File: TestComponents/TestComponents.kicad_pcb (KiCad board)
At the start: 2 copper layers, 101.7 x 73.7 mm, 119 parts, among them J2-1 Conn_01x04_Male, J2-2 Conn_01x04_Male, J3V1 Conn_01x01_Male, J5 RFShield_OnePiece, J6 RFShield_OnePiece, SW1 SW_SPDT, SW2 SW_SP3T, SW3 SW_SP3T, U1 AD7991, U13 X, U2 ADS1219, U3 REF200AU, U4 MCP6L01x-xLT, U8 ADR510, U9 LM4040B

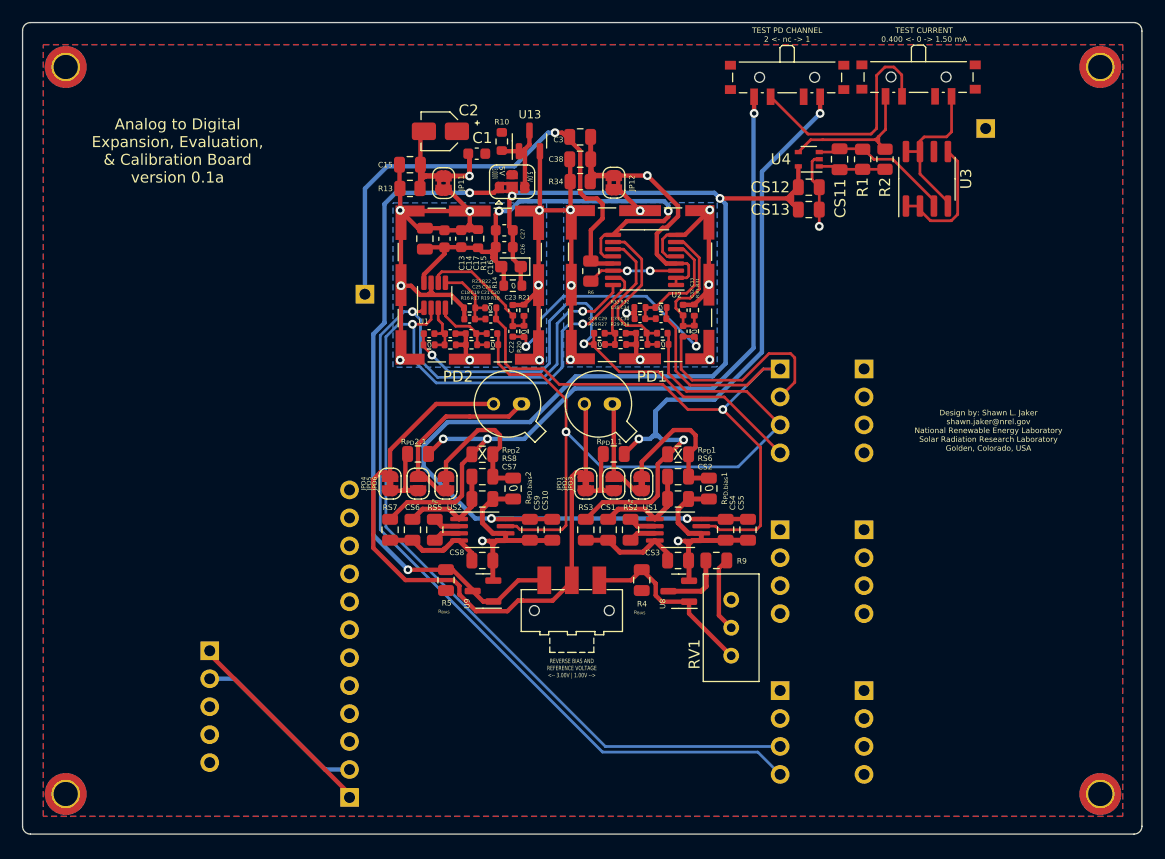
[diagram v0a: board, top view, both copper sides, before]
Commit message: SpectDrone Development
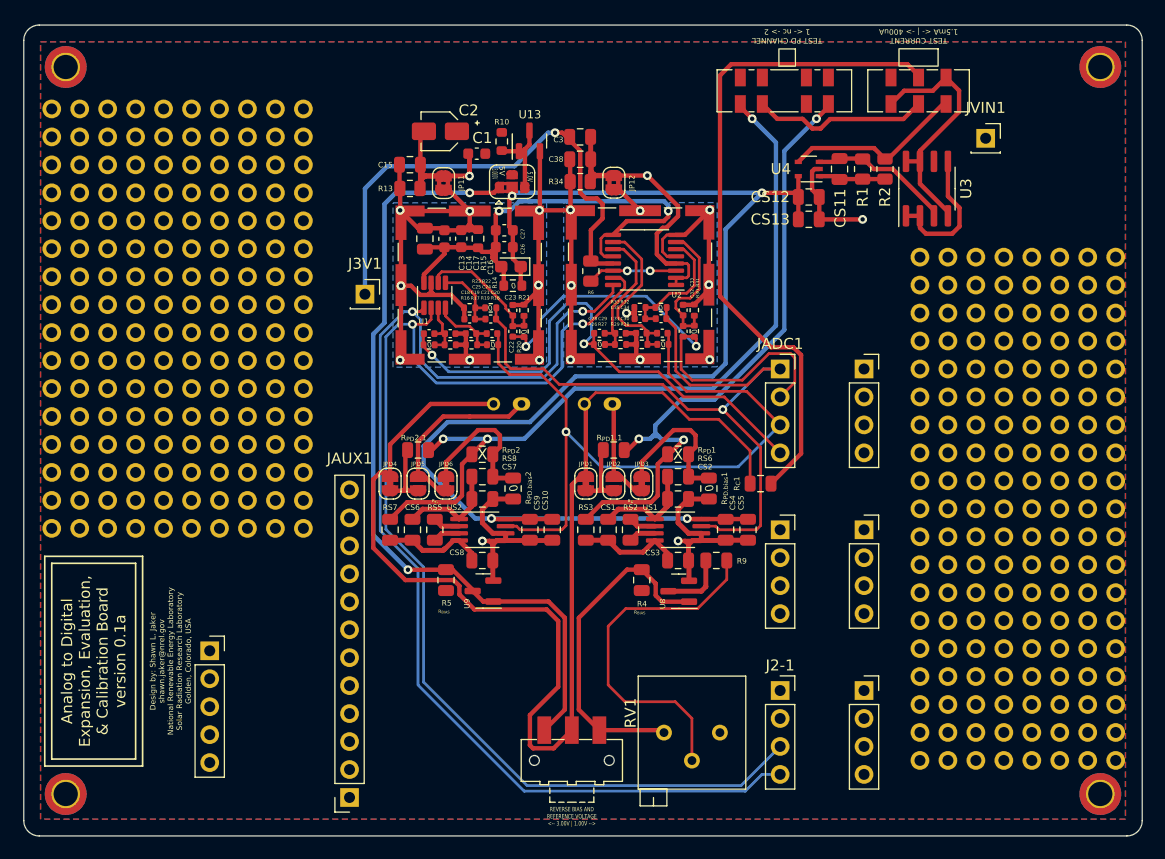
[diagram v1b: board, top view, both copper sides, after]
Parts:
- added REF**: TestPoint_THTPad_D2.0mm_Drill1.0mm, TestPoint:TestPoint_THTPad_D2.0mm_Drill1.0mm, F.Cu at (105.4, 73.7)
- added REF**: TestPoint_THTPad_D2.0mm_Drill1.0mm, TestPoint:TestPoint_THTPad_D2.0mm_Drill1.0mm, F.Cu at (184.3, 87.1)
- added REF**1: TestPoint_THTPad_D2.0mm_Drill1.0mm, TestPoint:TestPoint_THTPad_D2.0mm_Drill1.0mm, F.Cu at (108.0, 73.7)
- added REF**10: TestPoint_THTPad_D2.0mm_Drill1.0mm, TestPoint:TestPoint_THTPad_D2.0mm_Drill1.0mm, F.Cu at (105.4, 76.2)
- added REF**100: TestPoint_THTPad_D2.0mm_Drill1.0mm, TestPoint:TestPoint_THTPad_D2.0mm_Drill1.0mm, F.Cu at (105.4, 99.1)
- added REF**101: TestPoint_THTPad_D2.0mm_Drill1.0mm, TestPoint:TestPoint_THTPad_D2.0mm_Drill1.0mm, F.Cu at (108.0, 99.1)
- added REF**102: TestPoint_THTPad_D2.0mm_Drill1.0mm, TestPoint:TestPoint_THTPad_D2.0mm_Drill1.0mm, F.Cu at (110.5, 99.1)
- added REF**103: TestPoint_THTPad_D2.0mm_Drill1.0mm, TestPoint:TestPoint_THTPad_D2.0mm_Drill1.0mm, F.Cu at (113.0, 99.1)
- added REF**104: TestPoint_THTPad_D2.0mm_Drill1.0mm, TestPoint:TestPoint_THTPad_D2.0mm_Drill1.0mm, F.Cu at (115.6, 99.1)
- added REF**105: TestPoint_THTPad_D2.0mm_Drill1.0mm, TestPoint:TestPoint_THTPad_D2.0mm_Drill1.0mm, F.Cu at (118.1, 99.1)
- added REF**106: TestPoint_THTPad_D2.0mm_Drill1.0mm, TestPoint:TestPoint_THTPad_D2.0mm_Drill1.0mm, F.Cu at (120.7, 99.1)
- added REF**107: TestPoint_THTPad_D2.0mm_Drill1.0mm, TestPoint:TestPoint_THTPad_D2.0mm_Drill1.0mm, F.Cu at (123.2, 99.1)
- added REF**108: TestPoint_THTPad_D2.0mm_Drill1.0mm, TestPoint:TestPoint_THTPad_D2.0mm_Drill1.0mm, F.Cu at (125.7, 99.1)
- added REF**109: TestPoint_THTPad_D2.0mm_Drill1.0mm, TestPoint:TestPoint_THTPad_D2.0mm_Drill1.0mm, F.Cu at (128.3, 99.1)
- added REF**11: TestPoint_THTPad_D2.0mm_Drill1.0mm, TestPoint:TestPoint_THTPad_D2.0mm_Drill1.0mm, F.Cu at (108.0, 76.2)
- added REF**110: TestPoint_THTPad_D2.0mm_Drill1.0mm, TestPoint:TestPoint_THTPad_D2.0mm_Drill1.0mm, F.Cu at (105.4, 101.6)
- added REF**111: TestPoint_THTPad_D2.0mm_Drill1.0mm, TestPoint:TestPoint_THTPad_D2.0mm_Drill1.0mm, F.Cu at (108.0, 101.6)
- added REF**112: TestPoint_THTPad_D2.0mm_Drill1.0mm, TestPoint:TestPoint_THTPad_D2.0mm_Drill1.0mm, F.Cu at (110.5, 101.6)
- added REF**113: TestPoint_THTPad_D2.0mm_Drill1.0mm, TestPoint:TestPoint_THTPad_D2.0mm_Drill1.0mm, F.Cu at (113.0, 101.6)
- added REF**114: TestPoint_THTPad_D2.0mm_Drill1.0mm, TestPoint:TestPoint_THTPad_D2.0mm_Drill1.0mm, F.Cu at (115.6, 101.6)
- added REF**115: TestPoint_THTPad_D2.0mm_Drill1.0mm, TestPoint:TestPoint_THTPad_D2.0mm_Drill1.0mm, F.Cu at (118.1, 101.6)
- added REF**116: TestPoint_THTPad_D2.0mm_Drill1.0mm, TestPoint:TestPoint_THTPad_D2.0mm_Drill1.0mm, F.Cu at (120.7, 101.6)
- added REF**117: TestPoint_THTPad_D2.0mm_Drill1.0mm, TestPoint:TestPoint_THTPad_D2.0mm_Drill1.0mm, F.Cu at (123.2, 101.6)
- added REF**118: TestPoint_THTPad_D2.0mm_Drill1.0mm, TestPoint:TestPoint_THTPad_D2.0mm_Drill1.0mm, F.Cu at (125.7, 101.6)
- added REF**119: TestPoint_THTPad_D2.0mm_Drill1.0mm, TestPoint:TestPoint_THTPad_D2.0mm_Drill1.0mm, F.Cu at (128.3, 101.6)
- added REF**12: TestPoint_THTPad_D2.0mm_Drill1.0mm, TestPoint:TestPoint_THTPad_D2.0mm_Drill1.0mm, F.Cu at (110.5, 76.2)
- added REF**120: TestPoint_THTPad_D2.0mm_Drill1.0mm, TestPoint:TestPoint_THTPad_D2.0mm_Drill1.0mm, F.Cu at (105.4, 104.1)
- added REF**121: TestPoint_THTPad_D2.0mm_Drill1.0mm, TestPoint:TestPoint_THTPad_D2.0mm_Drill1.0mm, F.Cu at (108.0, 104.1)
- added REF**122: TestPoint_THTPad_D2.0mm_Drill1.0mm, TestPoint:TestPoint_THTPad_D2.0mm_Drill1.0mm, F.Cu at (110.5, 104.1)
- added REF**123: TestPoint_THTPad_D2.0mm_Drill1.0mm, TestPoint:TestPoint_THTPad_D2.0mm_Drill1.0mm, F.Cu at (113.0, 104.1)
- added REF**124: TestPoint_THTPad_D2.0mm_Drill1.0mm, TestPoint:TestPoint_THTPad_D2.0mm_Drill1.0mm, F.Cu at (115.6, 104.1)
- added REF**125: TestPoint_THTPad_D2.0mm_Drill1.0mm, TestPoint:TestPoint_THTPad_D2.0mm_Drill1.0mm, F.Cu at (118.1, 104.1)
- added REF**126: TestPoint_THTPad_D2.0mm_Drill1.0mm, TestPoint:TestPoint_THTPad_D2.0mm_Drill1.0mm, F.Cu at (120.7, 104.1)
- added REF**127: TestPoint_THTPad_D2.0mm_Drill1.0mm, TestPoint:TestPoint_THTPad_D2.0mm_Drill1.0mm, F.Cu at (123.2, 104.1)
- added REF**128: TestPoint_THTPad_D2.0mm_Drill1.0mm, TestPoint:TestPoint_THTPad_D2.0mm_Drill1.0mm, F.Cu at (125.7, 104.1)
- added REF**129: TestPoint_THTPad_D2.0mm_Drill1.0mm, TestPoint:TestPoint_THTPad_D2.0mm_Drill1.0mm, F.Cu at (128.3, 104.1)
- added REF**13: TestPoint_THTPad_D2.0mm_Drill1.0mm, TestPoint:TestPoint_THTPad_D2.0mm_Drill1.0mm, F.Cu at (113.0, 76.2)
- added REF**130: TestPoint_THTPad_D2.0mm_Drill1.0mm, TestPoint:TestPoint_THTPad_D2.0mm_Drill1.0mm, F.Cu at (105.4, 106.7)
- added REF**131: TestPoint_THTPad_D2.0mm_Drill1.0mm, TestPoint:TestPoint_THTPad_D2.0mm_Drill1.0mm, F.Cu at (108.0, 106.7)
- added REF**132: TestPoint_THTPad_D2.0mm_Drill1.0mm, TestPoint:TestPoint_THTPad_D2.0mm_Drill1.0mm, F.Cu at (110.5, 106.7)
- added REF**133: TestPoint_THTPad_D2.0mm_Drill1.0mm, TestPoint:TestPoint_THTPad_D2.0mm_Drill1.0mm, F.Cu at (113.0, 106.7)
- added REF**134: TestPoint_THTPad_D2.0mm_Drill1.0mm, TestPoint:TestPoint_THTPad_D2.0mm_Drill1.0mm, F.Cu at (115.6, 106.7)
- added REF**135: TestPoint_THTPad_D2.0mm_Drill1.0mm, TestPoint:TestPoint_THTPad_D2.0mm_Drill1.0mm, F.Cu at (118.1, 106.7)
- added REF**136: TestPoint_THTPad_D2.0mm_Drill1.0mm, TestPoint:TestPoint_THTPad_D2.0mm_Drill1.0mm, F.Cu at (120.7, 106.7)
- added REF**137: TestPoint_THTPad_D2.0mm_Drill1.0mm, TestPoint:TestPoint_THTPad_D2.0mm_Drill1.0mm, F.Cu at (123.2, 106.7)
- added REF**138: TestPoint_THTPad_D2.0mm_Drill1.0mm, TestPoint:TestPoint_THTPad_D2.0mm_Drill1.0mm, F.Cu at (125.7, 106.7)
- added REF**139: TestPoint_THTPad_D2.0mm_Drill1.0mm, TestPoint:TestPoint_THTPad_D2.0mm_Drill1.0mm, F.Cu at (128.3, 106.7)
- added REF**14: TestPoint_THTPad_D2.0mm_Drill1.0mm, TestPoint:TestPoint_THTPad_D2.0mm_Drill1.0mm, F.Cu at (115.6, 76.2)
- added REF**140: TestPoint_THTPad_D2.0mm_Drill1.0mm, TestPoint:TestPoint_THTPad_D2.0mm_Drill1.0mm, F.Cu at (105.4, 109.2)
- added REF**141: TestPoint_THTPad_D2.0mm_Drill1.0mm, TestPoint:TestPoint_THTPad_D2.0mm_Drill1.0mm, F.Cu at (108.0, 109.2)
- added REF**142: TestPoint_THTPad_D2.0mm_Drill1.0mm, TestPoint:TestPoint_THTPad_D2.0mm_Drill1.0mm, F.Cu at (110.5, 109.2)
- added REF**143: TestPoint_THTPad_D2.0mm_Drill1.0mm, TestPoint:TestPoint_THTPad_D2.0mm_Drill1.0mm, F.Cu at (113.0, 109.2)
- added REF**144: TestPoint_THTPad_D2.0mm_Drill1.0mm, TestPoint:TestPoint_THTPad_D2.0mm_Drill1.0mm, F.Cu at (115.6, 109.2)
- added REF**145: TestPoint_THTPad_D2.0mm_Drill1.0mm, TestPoint:TestPoint_THTPad_D2.0mm_Drill1.0mm, F.Cu at (118.1, 109.2)
- added REF**146: TestPoint_THTPad_D2.0mm_Drill1.0mm, TestPoint:TestPoint_THTPad_D2.0mm_Drill1.0mm, F.Cu at (120.7, 109.2)
- added REF**147: TestPoint_THTPad_D2.0mm_Drill1.0mm, TestPoint:TestPoint_THTPad_D2.0mm_Drill1.0mm, F.Cu at (123.2, 109.2)
- added REF**148: TestPoint_THTPad_D2.0mm_Drill1.0mm, TestPoint:TestPoint_THTPad_D2.0mm_Drill1.0mm, F.Cu at (125.7, 109.2)
- added REF**149: TestPoint_THTPad_D2.0mm_Drill1.0mm, TestPoint:TestPoint_THTPad_D2.0mm_Drill1.0mm, F.Cu at (128.3, 109.2)
- added REF**15: TestPoint_THTPad_D2.0mm_Drill1.0mm, TestPoint:TestPoint_THTPad_D2.0mm_Drill1.0mm, F.Cu at (118.1, 76.2)
- added REF**150: TestPoint_THTPad_D2.0mm_Drill1.0mm, TestPoint:TestPoint_THTPad_D2.0mm_Drill1.0mm, F.Cu at (105.4, 111.8)
- added REF**151: TestPoint_THTPad_D2.0mm_Drill1.0mm, TestPoint:TestPoint_THTPad_D2.0mm_Drill1.0mm, F.Cu at (108.0, 111.8)
- added REF**152: TestPoint_THTPad_D2.0mm_Drill1.0mm, TestPoint:TestPoint_THTPad_D2.0mm_Drill1.0mm, F.Cu at (110.5, 111.8)
- added REF**153: TestPoint_THTPad_D2.0mm_Drill1.0mm, TestPoint:TestPoint_THTPad_D2.0mm_Drill1.0mm, F.Cu at (113.0, 111.8)
- added REF**154: TestPoint_THTPad_D2.0mm_Drill1.0mm, TestPoint:TestPoint_THTPad_D2.0mm_Drill1.0mm, F.Cu at (115.6, 111.8)
- added REF**155: TestPoint_THTPad_D2.0mm_Drill1.0mm, TestPoint:TestPoint_THTPad_D2.0mm_Drill1.0mm, F.Cu at (118.1, 111.8)
- added REF**156: TestPoint_THTPad_D2.0mm_Drill1.0mm, TestPoint:TestPoint_THTPad_D2.0mm_Drill1.0mm, F.Cu at (120.7, 111.8)
- added REF**157: TestPoint_THTPad_D2.0mm_Drill1.0mm, TestPoint:TestPoint_THTPad_D2.0mm_Drill1.0mm, F.Cu at (123.2, 111.8)
- added REF**158: TestPoint_THTPad_D2.0mm_Drill1.0mm, TestPoint:TestPoint_THTPad_D2.0mm_Drill1.0mm, F.Cu at (125.7, 111.8)
- added REF**159: TestPoint_THTPad_D2.0mm_Drill1.0mm, TestPoint:TestPoint_THTPad_D2.0mm_Drill1.0mm, F.Cu at (128.3, 111.8)
- added REF**16: TestPoint_THTPad_D2.0mm_Drill1.0mm, TestPoint:TestPoint_THTPad_D2.0mm_Drill1.0mm, F.Cu at (120.7, 76.2)
- added REF**160: TestPoint_THTPad_D2.0mm_Drill1.0mm, TestPoint:TestPoint_THTPad_D2.0mm_Drill1.0mm, F.Cu at (186.8, 87.1)
- added REF**161: TestPoint_THTPad_D2.0mm_Drill1.0mm, TestPoint:TestPoint_THTPad_D2.0mm_Drill1.0mm, F.Cu at (189.4, 87.1)
- added REF**162: TestPoint_THTPad_D2.0mm_Drill1.0mm, TestPoint:TestPoint_THTPad_D2.0mm_Drill1.0mm, F.Cu at (191.9, 87.1)
- added REF**163: TestPoint_THTPad_D2.0mm_Drill1.0mm, TestPoint:TestPoint_THTPad_D2.0mm_Drill1.0mm, F.Cu at (194.4, 87.1)
- added REF**164: TestPoint_THTPad_D2.0mm_Drill1.0mm, TestPoint:TestPoint_THTPad_D2.0mm_Drill1.0mm, F.Cu at (197.0, 87.1)
- added REF**165: TestPoint_THTPad_D2.0mm_Drill1.0mm, TestPoint:TestPoint_THTPad_D2.0mm_Drill1.0mm, F.Cu at (199.5, 87.1)
- added REF**166: TestPoint_THTPad_D2.0mm_Drill1.0mm, TestPoint:TestPoint_THTPad_D2.0mm_Drill1.0mm, F.Cu at (202.1, 87.1)
- added REF**167: TestPoint_THTPad_D2.0mm_Drill1.0mm, TestPoint:TestPoint_THTPad_D2.0mm_Drill1.0mm, F.Cu at (184.3, 89.7)
- added REF**168: TestPoint_THTPad_D2.0mm_Drill1.0mm, TestPoint:TestPoint_THTPad_D2.0mm_Drill1.0mm, F.Cu at (186.8, 89.7)
- added REF**169: TestPoint_THTPad_D2.0mm_Drill1.0mm, TestPoint:TestPoint_THTPad_D2.0mm_Drill1.0mm, F.Cu at (189.4, 89.7)
- added REF**17: TestPoint_THTPad_D2.0mm_Drill1.0mm, TestPoint:TestPoint_THTPad_D2.0mm_Drill1.0mm, F.Cu at (123.2, 76.2)
- added REF**170: TestPoint_THTPad_D2.0mm_Drill1.0mm, TestPoint:TestPoint_THTPad_D2.0mm_Drill1.0mm, F.Cu at (191.9, 89.7)
- added REF**171: TestPoint_THTPad_D2.0mm_Drill1.0mm, TestPoint:TestPoint_THTPad_D2.0mm_Drill1.0mm, F.Cu at (194.4, 89.7)
- added REF**172: TestPoint_THTPad_D2.0mm_Drill1.0mm, TestPoint:TestPoint_THTPad_D2.0mm_Drill1.0mm, F.Cu at (197.0, 89.7)
- added REF**173: TestPoint_THTPad_D2.0mm_Drill1.0mm, TestPoint:TestPoint_THTPad_D2.0mm_Drill1.0mm, F.Cu at (199.5, 89.7)
- added REF**174: TestPoint_THTPad_D2.0mm_Drill1.0mm, TestPoint:TestPoint_THTPad_D2.0mm_Drill1.0mm, F.Cu at (202.1, 89.7)
- added REF**175: TestPoint_THTPad_D2.0mm_Drill1.0mm, TestPoint:TestPoint_THTPad_D2.0mm_Drill1.0mm, F.Cu at (184.3, 92.2)
- added REF**176: TestPoint_THTPad_D2.0mm_Drill1.0mm, TestPoint:TestPoint_THTPad_D2.0mm_Drill1.0mm, F.Cu at (186.8, 92.2)
- added REF**177: TestPoint_THTPad_D2.0mm_Drill1.0mm, TestPoint:TestPoint_THTPad_D2.0mm_Drill1.0mm, F.Cu at (189.4, 92.2)
- added REF**178: TestPoint_THTPad_D2.0mm_Drill1.0mm, TestPoint:TestPoint_THTPad_D2.0mm_Drill1.0mm, F.Cu at (191.9, 92.2)
- added REF**179: TestPoint_THTPad_D2.0mm_Drill1.0mm, TestPoint:TestPoint_THTPad_D2.0mm_Drill1.0mm, F.Cu at (194.4, 92.2)
- added REF**18: TestPoint_THTPad_D2.0mm_Drill1.0mm, TestPoint:TestPoint_THTPad_D2.0mm_Drill1.0mm, F.Cu at (125.7, 76.2)
- added REF**180: TestPoint_THTPad_D2.0mm_Drill1.0mm, TestPoint:TestPoint_THTPad_D2.0mm_Drill1.0mm, F.Cu at (197.0, 92.2)
- added REF**181: TestPoint_THTPad_D2.0mm_Drill1.0mm, TestPoint:TestPoint_THTPad_D2.0mm_Drill1.0mm, F.Cu at (199.5, 92.2)
- added REF**182: TestPoint_THTPad_D2.0mm_Drill1.0mm, TestPoint:TestPoint_THTPad_D2.0mm_Drill1.0mm, F.Cu at (202.1, 92.2)
- added REF**183: TestPoint_THTPad_D2.0mm_Drill1.0mm, TestPoint:TestPoint_THTPad_D2.0mm_Drill1.0mm, F.Cu at (184.3, 94.7)
- added REF**184: TestPoint_THTPad_D2.0mm_Drill1.0mm, TestPoint:TestPoint_THTPad_D2.0mm_Drill1.0mm, F.Cu at (186.8, 94.7)
- added REF**185: TestPoint_THTPad_D2.0mm_Drill1.0mm, TestPoint:TestPoint_THTPad_D2.0mm_Drill1.0mm, F.Cu at (189.4, 94.7)
- added REF**186: TestPoint_THTPad_D2.0mm_Drill1.0mm, TestPoint:TestPoint_THTPad_D2.0mm_Drill1.0mm, F.Cu at (191.9, 94.7)
- added REF**187: TestPoint_THTPad_D2.0mm_Drill1.0mm, TestPoint:TestPoint_THTPad_D2.0mm_Drill1.0mm, F.Cu at (194.4, 94.7)
- added REF**188: TestPoint_THTPad_D2.0mm_Drill1.0mm, TestPoint:TestPoint_THTPad_D2.0mm_Drill1.0mm, F.Cu at (197.0, 94.7)
- added REF**189: TestPoint_THTPad_D2.0mm_Drill1.0mm, TestPoint:TestPoint_THTPad_D2.0mm_Drill1.0mm, F.Cu at (199.5, 94.7)
- added REF**19: TestPoint_THTPad_D2.0mm_Drill1.0mm, TestPoint:TestPoint_THTPad_D2.0mm_Drill1.0mm, F.Cu at (128.3, 76.2)
- added REF**190: TestPoint_THTPad_D2.0mm_Drill1.0mm, TestPoint:TestPoint_THTPad_D2.0mm_Drill1.0mm, F.Cu at (202.1, 94.7)
- added REF**191: TestPoint_THTPad_D2.0mm_Drill1.0mm, TestPoint:TestPoint_THTPad_D2.0mm_Drill1.0mm, F.Cu at (184.3, 97.3)
- added REF**192: TestPoint_THTPad_D2.0mm_Drill1.0mm, TestPoint:TestPoint_THTPad_D2.0mm_Drill1.0mm, F.Cu at (186.8, 97.3)
- added REF**193: TestPoint_THTPad_D2.0mm_Drill1.0mm, TestPoint:TestPoint_THTPad_D2.0mm_Drill1.0mm, F.Cu at (189.4, 97.3)
- added REF**194: TestPoint_THTPad_D2.0mm_Drill1.0mm, TestPoint:TestPoint_THTPad_D2.0mm_Drill1.0mm, F.Cu at (191.9, 97.3)
- added REF**195: TestPoint_THTPad_D2.0mm_Drill1.0mm, TestPoint:TestPoint_THTPad_D2.0mm_Drill1.0mm, F.Cu at (194.4, 97.3)
- added REF**196: TestPoint_THTPad_D2.0mm_Drill1.0mm, TestPoint:TestPoint_THTPad_D2.0mm_Drill1.0mm, F.Cu at (197.0, 97.3)
- added REF**197: TestPoint_THTPad_D2.0mm_Drill1.0mm, TestPoint:TestPoint_THTPad_D2.0mm_Drill1.0mm, F.Cu at (199.5, 97.3)
- added REF**198: TestPoint_THTPad_D2.0mm_Drill1.0mm, TestPoint:TestPoint_THTPad_D2.0mm_Drill1.0mm, F.Cu at (202.1, 97.3)
- added REF**199: TestPoint_THTPad_D2.0mm_Drill1.0mm, TestPoint:TestPoint_THTPad_D2.0mm_Drill1.0mm, F.Cu at (184.3, 99.8)
- added REF**2: TestPoint_THTPad_D2.0mm_Drill1.0mm, TestPoint:TestPoint_THTPad_D2.0mm_Drill1.0mm, F.Cu at (110.5, 73.7)
- added REF**20: TestPoint_THTPad_D2.0mm_Drill1.0mm, TestPoint:TestPoint_THTPad_D2.0mm_Drill1.0mm, F.Cu at (105.4, 78.7)
- added REF**200: TestPoint_THTPad_D2.0mm_Drill1.0mm, TestPoint:TestPoint_THTPad_D2.0mm_Drill1.0mm, F.Cu at (186.8, 99.8)
- added REF**201: TestPoint_THTPad_D2.0mm_Drill1.0mm, TestPoint:TestPoint_THTPad_D2.0mm_Drill1.0mm, F.Cu at (189.4, 99.8)
- added REF**202: TestPoint_THTPad_D2.0mm_Drill1.0mm, TestPoint:TestPoint_THTPad_D2.0mm_Drill1.0mm, F.Cu at (191.9, 99.8)
- added REF**203: TestPoint_THTPad_D2.0mm_Drill1.0mm, TestPoint:TestPoint_THTPad_D2.0mm_Drill1.0mm, F.Cu at (194.4, 99.8)
- added REF**204: TestPoint_THTPad_D2.0mm_Drill1.0mm, TestPoint:TestPoint_THTPad_D2.0mm_Drill1.0mm, F.Cu at (197.0, 99.8)
- added REF**205: TestPoint_THTPad_D2.0mm_Drill1.0mm, TestPoint:TestPoint_THTPad_D2.0mm_Drill1.0mm, F.Cu at (199.5, 99.8)
- added REF**206: TestPoint_THTPad_D2.0mm_Drill1.0mm, TestPoint:TestPoint_THTPad_D2.0mm_Drill1.0mm, F.Cu at (202.1, 99.8)
- added REF**207: TestPoint_THTPad_D2.0mm_Drill1.0mm, TestPoint:TestPoint_THTPad_D2.0mm_Drill1.0mm, F.Cu at (184.3, 102.4)
- added REF**208: TestPoint_THTPad_D2.0mm_Drill1.0mm, TestPoint:TestPoint_THTPad_D2.0mm_Drill1.0mm, F.Cu at (186.8, 102.4)
- added REF**209: TestPoint_THTPad_D2.0mm_Drill1.0mm, TestPoint:TestPoint_THTPad_D2.0mm_Drill1.0mm, F.Cu at (189.4, 102.4)
- added REF**21: TestPoint_THTPad_D2.0mm_Drill1.0mm, TestPoint:TestPoint_THTPad_D2.0mm_Drill1.0mm, F.Cu at (108.0, 78.7)
- added REF**210: TestPoint_THTPad_D2.0mm_Drill1.0mm, TestPoint:TestPoint_THTPad_D2.0mm_Drill1.0mm, F.Cu at (191.9, 102.4)
- added REF**211: TestPoint_THTPad_D2.0mm_Drill1.0mm, TestPoint:TestPoint_THTPad_D2.0mm_Drill1.0mm, F.Cu at (194.4, 102.4)
- added REF**212: TestPoint_THTPad_D2.0mm_Drill1.0mm, TestPoint:TestPoint_THTPad_D2.0mm_Drill1.0mm, F.Cu at (197.0, 102.4)
- added REF**213: TestPoint_THTPad_D2.0mm_Drill1.0mm, TestPoint:TestPoint_THTPad_D2.0mm_Drill1.0mm, F.Cu at (199.5, 102.4)
- added REF**214: TestPoint_THTPad_D2.0mm_Drill1.0mm, TestPoint:TestPoint_THTPad_D2.0mm_Drill1.0mm, F.Cu at (202.1, 102.4)
- added REF**215: TestPoint_THTPad_D2.0mm_Drill1.0mm, TestPoint:TestPoint_THTPad_D2.0mm_Drill1.0mm, F.Cu at (184.3, 104.9)
- added REF**216: TestPoint_THTPad_D2.0mm_Drill1.0mm, TestPoint:TestPoint_THTPad_D2.0mm_Drill1.0mm, F.Cu at (186.8, 104.9)
- added REF**217: TestPoint_THTPad_D2.0mm_Drill1.0mm, TestPoint:TestPoint_THTPad_D2.0mm_Drill1.0mm, F.Cu at (189.4, 104.9)
- added REF**218: TestPoint_THTPad_D2.0mm_Drill1.0mm, TestPoint:TestPoint_THTPad_D2.0mm_Drill1.0mm, F.Cu at (191.9, 104.9)
- added REF**219: TestPoint_THTPad_D2.0mm_Drill1.0mm, TestPoint:TestPoint_THTPad_D2.0mm_Drill1.0mm, F.Cu at (194.4, 104.9)
- added REF**22: TestPoint_THTPad_D2.0mm_Drill1.0mm, TestPoint:TestPoint_THTPad_D2.0mm_Drill1.0mm, F.Cu at (110.5, 78.7)
- added REF**220: TestPoint_THTPad_D2.0mm_Drill1.0mm, TestPoint:TestPoint_THTPad_D2.0mm_Drill1.0mm, F.Cu at (197.0, 104.9)
- added REF**221: TestPoint_THTPad_D2.0mm_Drill1.0mm, TestPoint:TestPoint_THTPad_D2.0mm_Drill1.0mm, F.Cu at (199.5, 104.9)
- added REF**222: TestPoint_THTPad_D2.0mm_Drill1.0mm, TestPoint:TestPoint_THTPad_D2.0mm_Drill1.0mm, F.Cu at (202.1, 104.9)
- added REF**223: TestPoint_THTPad_D2.0mm_Drill1.0mm, TestPoint:TestPoint_THTPad_D2.0mm_Drill1.0mm, F.Cu at (184.3, 107.4)
- added REF**224: TestPoint_THTPad_D2.0mm_Drill1.0mm, TestPoint:TestPoint_THTPad_D2.0mm_Drill1.0mm, F.Cu at (186.8, 107.4)
- added REF**225: TestPoint_THTPad_D2.0mm_Drill1.0mm, TestPoint:TestPoint_THTPad_D2.0mm_Drill1.0mm, F.Cu at (189.4, 107.4)
- added REF**226: TestPoint_THTPad_D2.0mm_Drill1.0mm, TestPoint:TestPoint_THTPad_D2.0mm_Drill1.0mm, F.Cu at (191.9, 107.4)
- added REF**227: TestPoint_THTPad_D2.0mm_Drill1.0mm, TestPoint:TestPoint_THTPad_D2.0mm_Drill1.0mm, F.Cu at (194.4, 107.4)
- added REF**228: TestPoint_THTPad_D2.0mm_Drill1.0mm, TestPoint:TestPoint_THTPad_D2.0mm_Drill1.0mm, F.Cu at (197.0, 107.4)
- added REF**229: TestPoint_THTPad_D2.0mm_Drill1.0mm, TestPoint:TestPoint_THTPad_D2.0mm_Drill1.0mm, F.Cu at (199.5, 107.4)
- added REF**23: TestPoint_THTPad_D2.0mm_Drill1.0mm, TestPoint:TestPoint_THTPad_D2.0mm_Drill1.0mm, F.Cu at (113.0, 78.7)
- added REF**230: TestPoint_THTPad_D2.0mm_Drill1.0mm, TestPoint:TestPoint_THTPad_D2.0mm_Drill1.0mm, F.Cu at (202.1, 107.4)
- added REF**231: TestPoint_THTPad_D2.0mm_Drill1.0mm, TestPoint:TestPoint_THTPad_D2.0mm_Drill1.0mm, F.Cu at (184.3, 110.0)
- added REF**232: TestPoint_THTPad_D2.0mm_Drill1.0mm, TestPoint:TestPoint_THTPad_D2.0mm_Drill1.0mm, F.Cu at (186.8, 110.0)
- added REF**233: TestPoint_THTPad_D2.0mm_Drill1.0mm, TestPoint:TestPoint_THTPad_D2.0mm_Drill1.0mm, F.Cu at (189.4, 110.0)
- added REF**234: TestPoint_THTPad_D2.0mm_Drill1.0mm, TestPoint:TestPoint_THTPad_D2.0mm_Drill1.0mm, F.Cu at (191.9, 110.0)
- added REF**235: TestPoint_THTPad_D2.0mm_Drill1.0mm, TestPoint:TestPoint_THTPad_D2.0mm_Drill1.0mm, F.Cu at (194.4, 110.0)
- added REF**236: TestPoint_THTPad_D2.0mm_Drill1.0mm, TestPoint:TestPoint_THTPad_D2.0mm_Drill1.0mm, F.Cu at (197.0, 110.0)
- added REF**237: TestPoint_THTPad_D2.0mm_Drill1.0mm, TestPoint:TestPoint_THTPad_D2.0mm_Drill1.0mm, F.Cu at (199.5, 110.0)
- added REF**238: TestPoint_THTPad_D2.0mm_Drill1.0mm, TestPoint:TestPoint_THTPad_D2.0mm_Drill1.0mm, F.Cu at (202.1, 110.0)
- added REF**239: TestPoint_THTPad_D2.0mm_Drill1.0mm, TestPoint:TestPoint_THTPad_D2.0mm_Drill1.0mm, F.Cu at (184.3, 112.5)
- added REF**24: TestPoint_THTPad_D2.0mm_Drill1.0mm, TestPoint:TestPoint_THTPad_D2.0mm_Drill1.0mm, F.Cu at (115.6, 78.7)
- added REF**240: TestPoint_THTPad_D2.0mm_Drill1.0mm, TestPoint:TestPoint_THTPad_D2.0mm_Drill1.0mm, F.Cu at (186.8, 112.5)
- added REF**241: TestPoint_THTPad_D2.0mm_Drill1.0mm, TestPoint:TestPoint_THTPad_D2.0mm_Drill1.0mm, F.Cu at (189.4, 112.5)
- added REF**242: TestPoint_THTPad_D2.0mm_Drill1.0mm, TestPoint:TestPoint_THTPad_D2.0mm_Drill1.0mm, F.Cu at (191.9, 112.5)
- added REF**243: TestPoint_THTPad_D2.0mm_Drill1.0mm, TestPoint:TestPoint_THTPad_D2.0mm_Drill1.0mm, F.Cu at (194.4, 112.5)
- added REF**244: TestPoint_THTPad_D2.0mm_Drill1.0mm, TestPoint:TestPoint_THTPad_D2.0mm_Drill1.0mm, F.Cu at (197.0, 112.5)
- added REF**245: TestPoint_THTPad_D2.0mm_Drill1.0mm, TestPoint:TestPoint_THTPad_D2.0mm_Drill1.0mm, F.Cu at (199.5, 112.5)
- added REF**246: TestPoint_THTPad_D2.0mm_Drill1.0mm, TestPoint:TestPoint_THTPad_D2.0mm_Drill1.0mm, F.Cu at (202.1, 112.5)
- added REF**247: TestPoint_THTPad_D2.0mm_Drill1.0mm, TestPoint:TestPoint_THTPad_D2.0mm_Drill1.0mm, F.Cu at (184.3, 115.1)
- added REF**248: TestPoint_THTPad_D2.0mm_Drill1.0mm, TestPoint:TestPoint_THTPad_D2.0mm_Drill1.0mm, F.Cu at (186.8, 115.1)
- added REF**249: TestPoint_THTPad_D2.0mm_Drill1.0mm, TestPoint:TestPoint_THTPad_D2.0mm_Drill1.0mm, F.Cu at (189.4, 115.1)
- added REF**25: TestPoint_THTPad_D2.0mm_Drill1.0mm, TestPoint:TestPoint_THTPad_D2.0mm_Drill1.0mm, F.Cu at (118.1, 78.7)
- added REF**250: TestPoint_THTPad_D2.0mm_Drill1.0mm, TestPoint:TestPoint_THTPad_D2.0mm_Drill1.0mm, F.Cu at (191.9, 115.1)
- added REF**251: TestPoint_THTPad_D2.0mm_Drill1.0mm, TestPoint:TestPoint_THTPad_D2.0mm_Drill1.0mm, F.Cu at (194.4, 115.1)
- added REF**252: TestPoint_THTPad_D2.0mm_Drill1.0mm, TestPoint:TestPoint_THTPad_D2.0mm_Drill1.0mm, F.Cu at (197.0, 115.1)
- added REF**253: TestPoint_THTPad_D2.0mm_Drill1.0mm, TestPoint:TestPoint_THTPad_D2.0mm_Drill1.0mm, F.Cu at (199.5, 115.1)
- added REF**254: TestPoint_THTPad_D2.0mm_Drill1.0mm, TestPoint:TestPoint_THTPad_D2.0mm_Drill1.0mm, F.Cu at (202.1, 115.1)
- added REF**255: TestPoint_THTPad_D2.0mm_Drill1.0mm, TestPoint:TestPoint_THTPad_D2.0mm_Drill1.0mm, F.Cu at (184.3, 117.6)
- added REF**256: TestPoint_THTPad_D2.0mm_Drill1.0mm, TestPoint:TestPoint_THTPad_D2.0mm_Drill1.0mm, F.Cu at (186.8, 117.6)
- added REF**257: TestPoint_THTPad_D2.0mm_Drill1.0mm, TestPoint:TestPoint_THTPad_D2.0mm_Drill1.0mm, F.Cu at (189.4, 117.6)
- added REF**258: TestPoint_THTPad_D2.0mm_Drill1.0mm, TestPoint:TestPoint_THTPad_D2.0mm_Drill1.0mm, F.Cu at (191.9, 117.6)
- added REF**259: TestPoint_THTPad_D2.0mm_Drill1.0mm, TestPoint:TestPoint_THTPad_D2.0mm_Drill1.0mm, F.Cu at (194.4, 117.6)
- added REF**26: TestPoint_THTPad_D2.0mm_Drill1.0mm, TestPoint:TestPoint_THTPad_D2.0mm_Drill1.0mm, F.Cu at (120.7, 78.7)
- added REF**260: TestPoint_THTPad_D2.0mm_Drill1.0mm, TestPoint:TestPoint_THTPad_D2.0mm_Drill1.0mm, F.Cu at (197.0, 117.6)
- added REF**261: TestPoint_THTPad_D2.0mm_Drill1.0mm, TestPoint:TestPoint_THTPad_D2.0mm_Drill1.0mm, F.Cu at (199.5, 117.6)
- added REF**262: TestPoint_THTPad_D2.0mm_Drill1.0mm, TestPoint:TestPoint_THTPad_D2.0mm_Drill1.0mm, F.Cu at (202.1, 117.6)
- added REF**263: TestPoint_THTPad_D2.0mm_Drill1.0mm, TestPoint:TestPoint_THTPad_D2.0mm_Drill1.0mm, F.Cu at (184.3, 120.1)
- added REF**264: TestPoint_THTPad_D2.0mm_Drill1.0mm, TestPoint:TestPoint_THTPad_D2.0mm_Drill1.0mm, F.Cu at (186.8, 120.1)
- added REF**265: TestPoint_THTPad_D2.0mm_Drill1.0mm, TestPoint:TestPoint_THTPad_D2.0mm_Drill1.0mm, F.Cu at (189.4, 120.1)
- added REF**266: TestPoint_THTPad_D2.0mm_Drill1.0mm, TestPoint:TestPoint_THTPad_D2.0mm_Drill1.0mm, F.Cu at (191.9, 120.1)
- added REF**267: TestPoint_THTPad_D2.0mm_Drill1.0mm, TestPoint:TestPoint_THTPad_D2.0mm_Drill1.0mm, F.Cu at (194.4, 120.1)
- added REF**268: TestPoint_THTPad_D2.0mm_Drill1.0mm, TestPoint:TestPoint_THTPad_D2.0mm_Drill1.0mm, F.Cu at (197.0, 120.1)
- added REF**269: TestPoint_THTPad_D2.0mm_Drill1.0mm, TestPoint:TestPoint_THTPad_D2.0mm_Drill1.0mm, F.Cu at (199.5, 120.1)
- added REF**27: TestPoint_THTPad_D2.0mm_Drill1.0mm, TestPoint:TestPoint_THTPad_D2.0mm_Drill1.0mm, F.Cu at (123.2, 78.7)
- added REF**270: TestPoint_THTPad_D2.0mm_Drill1.0mm, TestPoint:TestPoint_THTPad_D2.0mm_Drill1.0mm, F.Cu at (202.1, 120.1)
- added REF**271: TestPoint_THTPad_D2.0mm_Drill1.0mm, TestPoint:TestPoint_THTPad_D2.0mm_Drill1.0mm, F.Cu at (184.3, 122.7)
- added REF**272: TestPoint_THTPad_D2.0mm_Drill1.0mm, TestPoint:TestPoint_THTPad_D2.0mm_Drill1.0mm, F.Cu at (186.8, 122.7)
- added REF**273: TestPoint_THTPad_D2.0mm_Drill1.0mm, TestPoint:TestPoint_THTPad_D2.0mm_Drill1.0mm, F.Cu at (189.4, 122.7)
- added REF**274: TestPoint_THTPad_D2.0mm_Drill1.0mm, TestPoint:TestPoint_THTPad_D2.0mm_Drill1.0mm, F.Cu at (191.9, 122.7)
- added REF**275: TestPoint_THTPad_D2.0mm_Drill1.0mm, TestPoint:TestPoint_THTPad_D2.0mm_Drill1.0mm, F.Cu at (194.4, 122.7)
- added REF**276: TestPoint_THTPad_D2.0mm_Drill1.0mm, TestPoint:TestPoint_THTPad_D2.0mm_Drill1.0mm, F.Cu at (197.0, 122.7)
- added REF**277: TestPoint_THTPad_D2.0mm_Drill1.0mm, TestPoint:TestPoint_THTPad_D2.0mm_Drill1.0mm, F.Cu at (199.5, 122.7)
- added REF**278: TestPoint_THTPad_D2.0mm_Drill1.0mm, TestPoint:TestPoint_THTPad_D2.0mm_Drill1.0mm, F.Cu at (202.1, 122.7)
- added REF**279: TestPoint_THTPad_D2.0mm_Drill1.0mm, TestPoint:TestPoint_THTPad_D2.0mm_Drill1.0mm, F.Cu at (184.3, 125.2)
- added REF**28: TestPoint_THTPad_D2.0mm_Drill1.0mm, TestPoint:TestPoint_THTPad_D2.0mm_Drill1.0mm, F.Cu at (125.7, 78.7)
- added REF**280: TestPoint_THTPad_D2.0mm_Drill1.0mm, TestPoint:TestPoint_THTPad_D2.0mm_Drill1.0mm, F.Cu at (186.8, 125.2)
- added REF**281: TestPoint_THTPad_D2.0mm_Drill1.0mm, TestPoint:TestPoint_THTPad_D2.0mm_Drill1.0mm, F.Cu at (189.4, 125.2)
- added REF**282: TestPoint_THTPad_D2.0mm_Drill1.0mm, TestPoint:TestPoint_THTPad_D2.0mm_Drill1.0mm, F.Cu at (191.9, 125.2)
- added REF**283: TestPoint_THTPad_D2.0mm_Drill1.0mm, TestPoint:TestPoint_THTPad_D2.0mm_Drill1.0mm, F.Cu at (194.4, 125.2)
- added REF**284: TestPoint_THTPad_D2.0mm_Drill1.0mm, TestPoint:TestPoint_THTPad_D2.0mm_Drill1.0mm, F.Cu at (197.0, 125.2)
- added REF**285: TestPoint_THTPad_D2.0mm_Drill1.0mm, TestPoint:TestPoint_THTPad_D2.0mm_Drill1.0mm, F.Cu at (199.5, 125.2)
- added REF**286: TestPoint_THTPad_D2.0mm_Drill1.0mm, TestPoint:TestPoint_THTPad_D2.0mm_Drill1.0mm, F.Cu at (202.1, 125.2)
- added REF**287: TestPoint_THTPad_D2.0mm_Drill1.0mm, TestPoint:TestPoint_THTPad_D2.0mm_Drill1.0mm, F.Cu at (184.3, 127.8)
- added REF**288: TestPoint_THTPad_D2.0mm_Drill1.0mm, TestPoint:TestPoint_THTPad_D2.0mm_Drill1.0mm, F.Cu at (186.8, 127.8)
- added REF**289: TestPoint_THTPad_D2.0mm_Drill1.0mm, TestPoint:TestPoint_THTPad_D2.0mm_Drill1.0mm, F.Cu at (189.4, 127.8)
- added REF**29: TestPoint_THTPad_D2.0mm_Drill1.0mm, TestPoint:TestPoint_THTPad_D2.0mm_Drill1.0mm, F.Cu at (128.3, 78.7)
- added REF**290: TestPoint_THTPad_D2.0mm_Drill1.0mm, TestPoint:TestPoint_THTPad_D2.0mm_Drill1.0mm, F.Cu at (191.9, 127.8)
- added REF**291: TestPoint_THTPad_D2.0mm_Drill1.0mm, TestPoint:TestPoint_THTPad_D2.0mm_Drill1.0mm, F.Cu at (194.4, 127.8)
- added REF**292: TestPoint_THTPad_D2.0mm_Drill1.0mm, TestPoint:TestPoint_THTPad_D2.0mm_Drill1.0mm, F.Cu at (197.0, 127.8)
- added REF**293: TestPoint_THTPad_D2.0mm_Drill1.0mm, TestPoint:TestPoint_THTPad_D2.0mm_Drill1.0mm, F.Cu at (199.5, 127.8)
- added REF**294: TestPoint_THTPad_D2.0mm_Drill1.0mm, TestPoint:TestPoint_THTPad_D2.0mm_Drill1.0mm, F.Cu at (202.1, 127.8)
- added REF**295: TestPoint_THTPad_D2.0mm_Drill1.0mm, TestPoint:TestPoint_THTPad_D2.0mm_Drill1.0mm, F.Cu at (184.3, 130.3)
- added REF**296: TestPoint_THTPad_D2.0mm_Drill1.0mm, TestPoint:TestPoint_THTPad_D2.0mm_Drill1.0mm, F.Cu at (186.8, 130.3)
- added REF**297: TestPoint_THTPad_D2.0mm_Drill1.0mm, TestPoint:TestPoint_THTPad_D2.0mm_Drill1.0mm, F.Cu at (189.4, 130.3)
- added REF**298: TestPoint_THTPad_D2.0mm_Drill1.0mm, TestPoint:TestPoint_THTPad_D2.0mm_Drill1.0mm, F.Cu at (191.9, 130.3)
- added REF**299: TestPoint_THTPad_D2.0mm_Drill1.0mm, TestPoint:TestPoint_THTPad_D2.0mm_Drill1.0mm, F.Cu at (194.4, 130.3)
- added REF**3: TestPoint_THTPad_D2.0mm_Drill1.0mm, TestPoint:TestPoint_THTPad_D2.0mm_Drill1.0mm, F.Cu at (113.0, 73.7)
- added REF**30: TestPoint_THTPad_D2.0mm_Drill1.0mm, TestPoint:TestPoint_THTPad_D2.0mm_Drill1.0mm, F.Cu at (105.4, 81.3)
- added REF**300: TestPoint_THTPad_D2.0mm_Drill1.0mm, TestPoint:TestPoint_THTPad_D2.0mm_Drill1.0mm, F.Cu at (197.0, 130.3)
- added REF**301: TestPoint_THTPad_D2.0mm_Drill1.0mm, TestPoint:TestPoint_THTPad_D2.0mm_Drill1.0mm, F.Cu at (199.5, 130.3)
- added REF**302: TestPoint_THTPad_D2.0mm_Drill1.0mm, TestPoint:TestPoint_THTPad_D2.0mm_Drill1.0mm, F.Cu at (202.1, 130.3)
- added REF**303: TestPoint_THTPad_D2.0mm_Drill1.0mm, TestPoint:TestPoint_THTPad_D2.0mm_Drill1.0mm, F.Cu at (184.3, 132.8)
- added REF**304: TestPoint_THTPad_D2.0mm_Drill1.0mm, TestPoint:TestPoint_THTPad_D2.0mm_Drill1.0mm, F.Cu at (186.8, 132.8)
- added REF**305: TestPoint_THTPad_D2.0mm_Drill1.0mm, TestPoint:TestPoint_THTPad_D2.0mm_Drill1.0mm, F.Cu at (189.4, 132.8)
- added REF**306: TestPoint_THTPad_D2.0mm_Drill1.0mm, TestPoint:TestPoint_THTPad_D2.0mm_Drill1.0mm, F.Cu at (191.9, 132.8)
- added REF**307: TestPoint_THTPad_D2.0mm_Drill1.0mm, TestPoint:TestPoint_THTPad_D2.0mm_Drill1.0mm, F.Cu at (194.4, 132.8)
- added REF**308: TestPoint_THTPad_D2.0mm_Drill1.0mm, TestPoint:TestPoint_THTPad_D2.0mm_Drill1.0mm, F.Cu at (197.0, 132.8)
- added REF**309: TestPoint_THTPad_D2.0mm_Drill1.0mm, TestPoint:TestPoint_THTPad_D2.0mm_Drill1.0mm, F.Cu at (199.5, 132.8)
- added REF**31: TestPoint_THTPad_D2.0mm_Drill1.0mm, TestPoint:TestPoint_THTPad_D2.0mm_Drill1.0mm, F.Cu at (108.0, 81.3)
- added REF**310: TestPoint_THTPad_D2.0mm_Drill1.0mm, TestPoint:TestPoint_THTPad_D2.0mm_Drill1.0mm, F.Cu at (202.1, 132.8)
- added REF**32: TestPoint_THTPad_D2.0mm_Drill1.0mm, TestPoint:TestPoint_THTPad_D2.0mm_Drill1.0mm, F.Cu at (110.5, 81.3)
- added REF**33: TestPoint_THTPad_D2.0mm_Drill1.0mm, TestPoint:TestPoint_THTPad_D2.0mm_Drill1.0mm, F.Cu at (113.0, 81.3)
- added REF**34: TestPoint_THTPad_D2.0mm_Drill1.0mm, TestPoint:TestPoint_THTPad_D2.0mm_Drill1.0mm, F.Cu at (115.6, 81.3)
- added REF**35: TestPoint_THTPad_D2.0mm_Drill1.0mm, TestPoint:TestPoint_THTPad_D2.0mm_Drill1.0mm, F.Cu at (118.1, 81.3)
- added REF**36: TestPoint_THTPad_D2.0mm_Drill1.0mm, TestPoint:TestPoint_THTPad_D2.0mm_Drill1.0mm, F.Cu at (120.7, 81.3)
- added REF**37: TestPoint_THTPad_D2.0mm_Drill1.0mm, TestPoint:TestPoint_THTPad_D2.0mm_Drill1.0mm, F.Cu at (123.2, 81.3)
- added REF**38: TestPoint_THTPad_D2.0mm_Drill1.0mm, TestPoint:TestPoint_THTPad_D2.0mm_Drill1.0mm, F.Cu at (125.7, 81.3)
- added REF**39: TestPoint_THTPad_D2.0mm_Drill1.0mm, TestPoint:TestPoint_THTPad_D2.0mm_Drill1.0mm, F.Cu at (128.3, 81.3)
- added REF**4: TestPoint_THTPad_D2.0mm_Drill1.0mm, TestPoint:TestPoint_THTPad_D2.0mm_Drill1.0mm, F.Cu at (115.6, 73.7)
- added REF**40: TestPoint_THTPad_D2.0mm_Drill1.0mm, TestPoint:TestPoint_THTPad_D2.0mm_Drill1.0mm, F.Cu at (105.4, 83.8)
- added REF**41: TestPoint_THTPad_D2.0mm_Drill1.0mm, TestPoint:TestPoint_THTPad_D2.0mm_Drill1.0mm, F.Cu at (108.0, 83.8)
- added REF**42: TestPoint_THTPad_D2.0mm_Drill1.0mm, TestPoint:TestPoint_THTPad_D2.0mm_Drill1.0mm, F.Cu at (110.5, 83.8)
- added REF**43: TestPoint_THTPad_D2.0mm_Drill1.0mm, TestPoint:TestPoint_THTPad_D2.0mm_Drill1.0mm, F.Cu at (113.0, 83.8)
- added REF**44: TestPoint_THTPad_D2.0mm_Drill1.0mm, TestPoint:TestPoint_THTPad_D2.0mm_Drill1.0mm, F.Cu at (115.6, 83.8)
- added REF**45: TestPoint_THTPad_D2.0mm_Drill1.0mm, TestPoint:TestPoint_THTPad_D2.0mm_Drill1.0mm, F.Cu at (118.1, 83.8)
- added REF**46: TestPoint_THTPad_D2.0mm_Drill1.0mm, TestPoint:TestPoint_THTPad_D2.0mm_Drill1.0mm, F.Cu at (120.7, 83.8)
- added REF**47: TestPoint_THTPad_D2.0mm_Drill1.0mm, TestPoint:TestPoint_THTPad_D2.0mm_Drill1.0mm, F.Cu at (123.2, 83.8)
- added REF**48: TestPoint_THTPad_D2.0mm_Drill1.0mm, TestPoint:TestPoint_THTPad_D2.0mm_Drill1.0mm, F.Cu at (125.7, 83.8)
- added REF**49: TestPoint_THTPad_D2.0mm_Drill1.0mm, TestPoint:TestPoint_THTPad_D2.0mm_Drill1.0mm, F.Cu at (128.3, 83.8)
- added REF**5: TestPoint_THTPad_D2.0mm_Drill1.0mm, TestPoint:TestPoint_THTPad_D2.0mm_Drill1.0mm, F.Cu at (118.1, 73.7)
- added REF**50: TestPoint_THTPad_D2.0mm_Drill1.0mm, TestPoint:TestPoint_THTPad_D2.0mm_Drill1.0mm, F.Cu at (105.4, 86.4)
- added REF**51: TestPoint_THTPad_D2.0mm_Drill1.0mm, TestPoint:TestPoint_THTPad_D2.0mm_Drill1.0mm, F.Cu at (108.0, 86.4)
- added REF**52: TestPoint_THTPad_D2.0mm_Drill1.0mm, TestPoint:TestPoint_THTPad_D2.0mm_Drill1.0mm, F.Cu at (110.5, 86.4)
- added REF**53: TestPoint_THTPad_D2.0mm_Drill1.0mm, TestPoint:TestPoint_THTPad_D2.0mm_Drill1.0mm, F.Cu at (113.0, 86.4)
- added REF**54: TestPoint_THTPad_D2.0mm_Drill1.0mm, TestPoint:TestPoint_THTPad_D2.0mm_Drill1.0mm, F.Cu at (115.6, 86.4)
- added REF**55: TestPoint_THTPad_D2.0mm_Drill1.0mm, TestPoint:TestPoint_THTPad_D2.0mm_Drill1.0mm, F.Cu at (118.1, 86.4)
- added REF**56: TestPoint_THTPad_D2.0mm_Drill1.0mm, TestPoint:TestPoint_THTPad_D2.0mm_Drill1.0mm, F.Cu at (120.7, 86.4)
- added REF**57: TestPoint_THTPad_D2.0mm_Drill1.0mm, TestPoint:TestPoint_THTPad_D2.0mm_Drill1.0mm, F.Cu at (123.2, 86.4)
- added REF**58: TestPoint_THTPad_D2.0mm_Drill1.0mm, TestPoint:TestPoint_THTPad_D2.0mm_Drill1.0mm, F.Cu at (125.7, 86.4)
- added REF**59: TestPoint_THTPad_D2.0mm_Drill1.0mm, TestPoint:TestPoint_THTPad_D2.0mm_Drill1.0mm, F.Cu at (128.3, 86.4)
- added REF**6: TestPoint_THTPad_D2.0mm_Drill1.0mm, TestPoint:TestPoint_THTPad_D2.0mm_Drill1.0mm, F.Cu at (120.7, 73.7)
- added REF**60: TestPoint_THTPad_D2.0mm_Drill1.0mm, TestPoint:TestPoint_THTPad_D2.0mm_Drill1.0mm, F.Cu at (105.4, 88.9)
- added REF**61: TestPoint_THTPad_D2.0mm_Drill1.0mm, TestPoint:TestPoint_THTPad_D2.0mm_Drill1.0mm, F.Cu at (108.0, 88.9)
- added REF**62: TestPoint_THTPad_D2.0mm_Drill1.0mm, TestPoint:TestPoint_THTPad_D2.0mm_Drill1.0mm, F.Cu at (110.5, 88.9)
- added REF**63: TestPoint_THTPad_D2.0mm_Drill1.0mm, TestPoint:TestPoint_THTPad_D2.0mm_Drill1.0mm, F.Cu at (113.0, 88.9)
- added REF**64: TestPoint_THTPad_D2.0mm_Drill1.0mm, TestPoint:TestPoint_THTPad_D2.0mm_Drill1.0mm, F.Cu at (115.6, 88.9)
- added REF**65: TestPoint_THTPad_D2.0mm_Drill1.0mm, TestPoint:TestPoint_THTPad_D2.0mm_Drill1.0mm, F.Cu at (118.1, 88.9)
- added REF**66: TestPoint_THTPad_D2.0mm_Drill1.0mm, TestPoint:TestPoint_THTPad_D2.0mm_Drill1.0mm, F.Cu at (120.7, 88.9)
- added REF**67: TestPoint_THTPad_D2.0mm_Drill1.0mm, TestPoint:TestPoint_THTPad_D2.0mm_Drill1.0mm, F.Cu at (123.2, 88.9)
- added REF**68: TestPoint_THTPad_D2.0mm_Drill1.0mm, TestPoint:TestPoint_THTPad_D2.0mm_Drill1.0mm, F.Cu at (125.7, 88.9)
- added REF**69: TestPoint_THTPad_D2.0mm_Drill1.0mm, TestPoint:TestPoint_THTPad_D2.0mm_Drill1.0mm, F.Cu at (128.3, 88.9)
- added REF**7: TestPoint_THTPad_D2.0mm_Drill1.0mm, TestPoint:TestPoint_THTPad_D2.0mm_Drill1.0mm, F.Cu at (123.2, 73.7)
- added REF**70: TestPoint_THTPad_D2.0mm_Drill1.0mm, TestPoint:TestPoint_THTPad_D2.0mm_Drill1.0mm, F.Cu at (105.4, 91.4)
- added REF**71: TestPoint_THTPad_D2.0mm_Drill1.0mm, TestPoint:TestPoint_THTPad_D2.0mm_Drill1.0mm, F.Cu at (108.0, 91.4)
- added REF**72: TestPoint_THTPad_D2.0mm_Drill1.0mm, TestPoint:TestPoint_THTPad_D2.0mm_Drill1.0mm, F.Cu at (110.5, 91.4)
- added REF**73: TestPoint_THTPad_D2.0mm_Drill1.0mm, TestPoint:TestPoint_THTPad_D2.0mm_Drill1.0mm, F.Cu at (113.0, 91.4)
- added REF**74: TestPoint_THTPad_D2.0mm_Drill1.0mm, TestPoint:TestPoint_THTPad_D2.0mm_Drill1.0mm, F.Cu at (115.6, 91.4)
- added REF**75: TestPoint_THTPad_D2.0mm_Drill1.0mm, TestPoint:TestPoint_THTPad_D2.0mm_Drill1.0mm, F.Cu at (118.1, 91.4)
- added REF**76: TestPoint_THTPad_D2.0mm_Drill1.0mm, TestPoint:TestPoint_THTPad_D2.0mm_Drill1.0mm, F.Cu at (120.7, 91.4)
- added REF**77: TestPoint_THTPad_D2.0mm_Drill1.0mm, TestPoint:TestPoint_THTPad_D2.0mm_Drill1.0mm, F.Cu at (123.2, 91.4)
- added REF**78: TestPoint_THTPad_D2.0mm_Drill1.0mm, TestPoint:TestPoint_THTPad_D2.0mm_Drill1.0mm, F.Cu at (125.7, 91.4)
- added REF**79: TestPoint_THTPad_D2.0mm_Drill1.0mm, TestPoint:TestPoint_THTPad_D2.0mm_Drill1.0mm, F.Cu at (128.3, 91.4)
- added REF**8: TestPoint_THTPad_D2.0mm_Drill1.0mm, TestPoint:TestPoint_THTPad_D2.0mm_Drill1.0mm, F.Cu at (125.7, 73.7)
- added REF**80: TestPoint_THTPad_D2.0mm_Drill1.0mm, TestPoint:TestPoint_THTPad_D2.0mm_Drill1.0mm, F.Cu at (105.4, 94.0)
- added REF**81: TestPoint_THTPad_D2.0mm_Drill1.0mm, TestPoint:TestPoint_THTPad_D2.0mm_Drill1.0mm, F.Cu at (108.0, 94.0)
- added REF**82: TestPoint_THTPad_D2.0mm_Drill1.0mm, TestPoint:TestPoint_THTPad_D2.0mm_Drill1.0mm, F.Cu at (110.5, 94.0)
- added REF**83: TestPoint_THTPad_D2.0mm_Drill1.0mm, TestPoint:TestPoint_THTPad_D2.0mm_Drill1.0mm, F.Cu at (113.0, 94.0)
- added REF**84: TestPoint_THTPad_D2.0mm_Drill1.0mm, TestPoint:TestPoint_THTPad_D2.0mm_Drill1.0mm, F.Cu at (115.6, 94.0)
- added REF**85: TestPoint_THTPad_D2.0mm_Drill1.0mm, TestPoint:TestPoint_THTPad_D2.0mm_Drill1.0mm, F.Cu at (118.1, 94.0)
- added REF**86: TestPoint_THTPad_D2.0mm_Drill1.0mm, TestPoint:TestPoint_THTPad_D2.0mm_Drill1.0mm, F.Cu at (120.7, 94.0)
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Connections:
- JGPS1 pad 1: /TestConnectors/5V -> /TestConnectors/GPS_5V
- JGPS1 pad 2: /TestConnectors/GND -> /TestConnectors/GPS_GND
- SW3 pad 1: -I_{const}=0.4mA -> -I_{const}=1.5mA
- SW3 pad 2: unconnected-(SW3-Pad2) -> /InsturmentationsAmps/PD_{TEST}
- SW3 pad 3: /InsturmentationsAmps/PD_{TEST} -> -I_{const}=0.4mA
- SW3 pad 4: -I_{const}=1.5mA -> -I_{const}=0.4mA
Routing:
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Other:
- board size 101.7 x 73.7 mm -> 101.6 x 73.7 mm
- board text added: "TEST CURRENT 1.5mA <- | -> 400uA"
- board text added: "TEST PD CHANNEL 1 <- nc -> 2"
- board text removed: "TEST CURRENT 0.400 <- 0 -> 1.50 mA"
- board text removed: "TEST PD CHANNEL 2 <- nc -> 1"
